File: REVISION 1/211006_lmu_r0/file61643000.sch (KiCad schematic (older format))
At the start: 7 parts

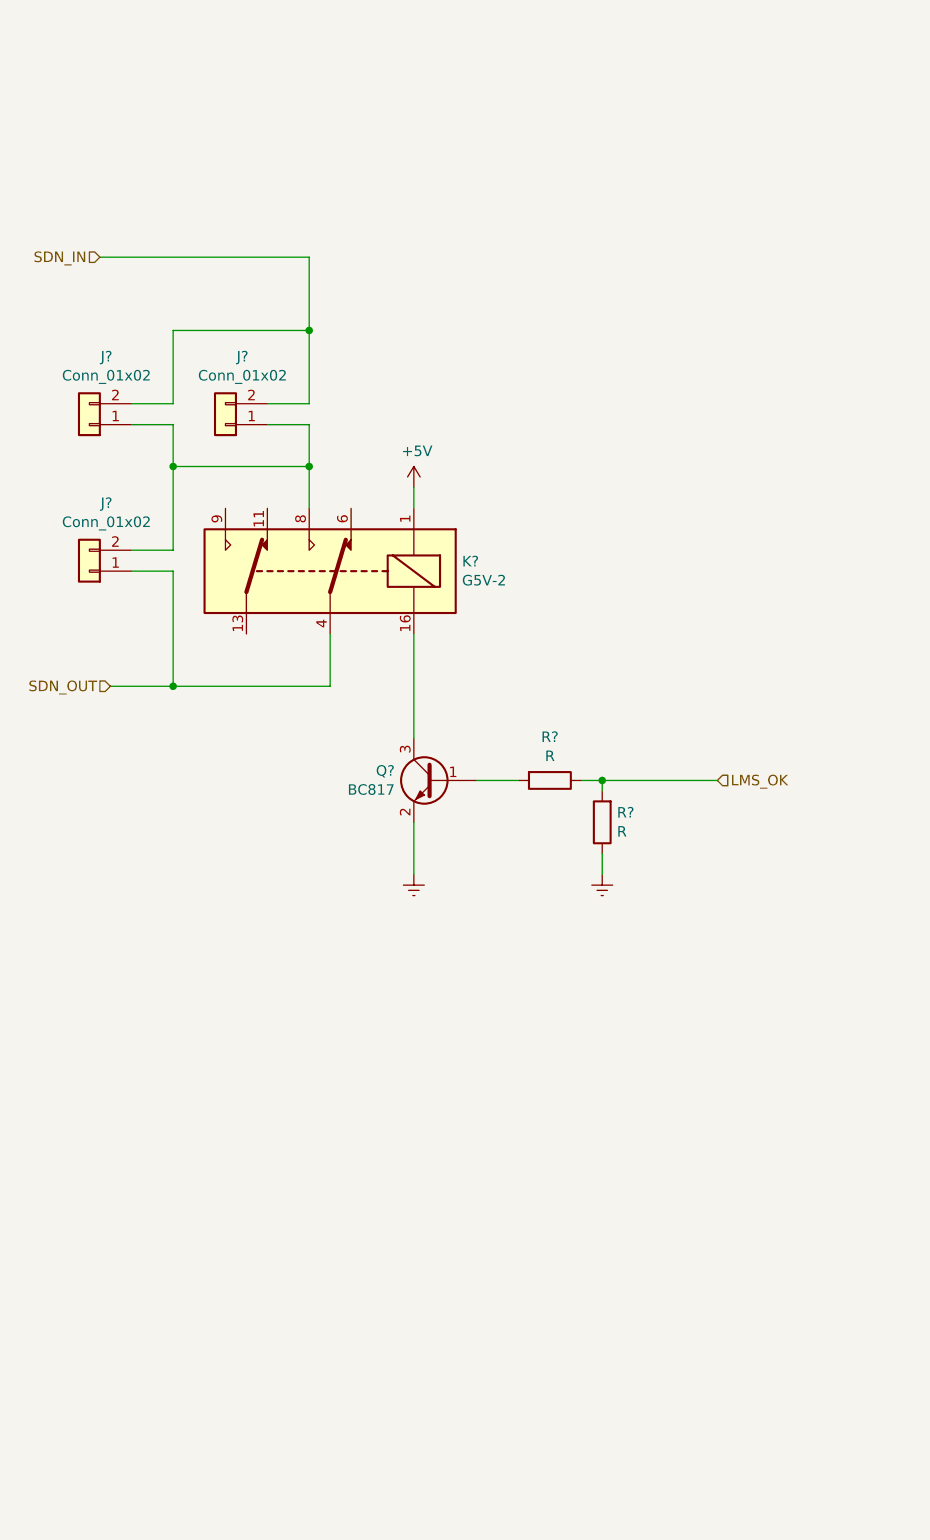
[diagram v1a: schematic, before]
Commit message: LMU design init
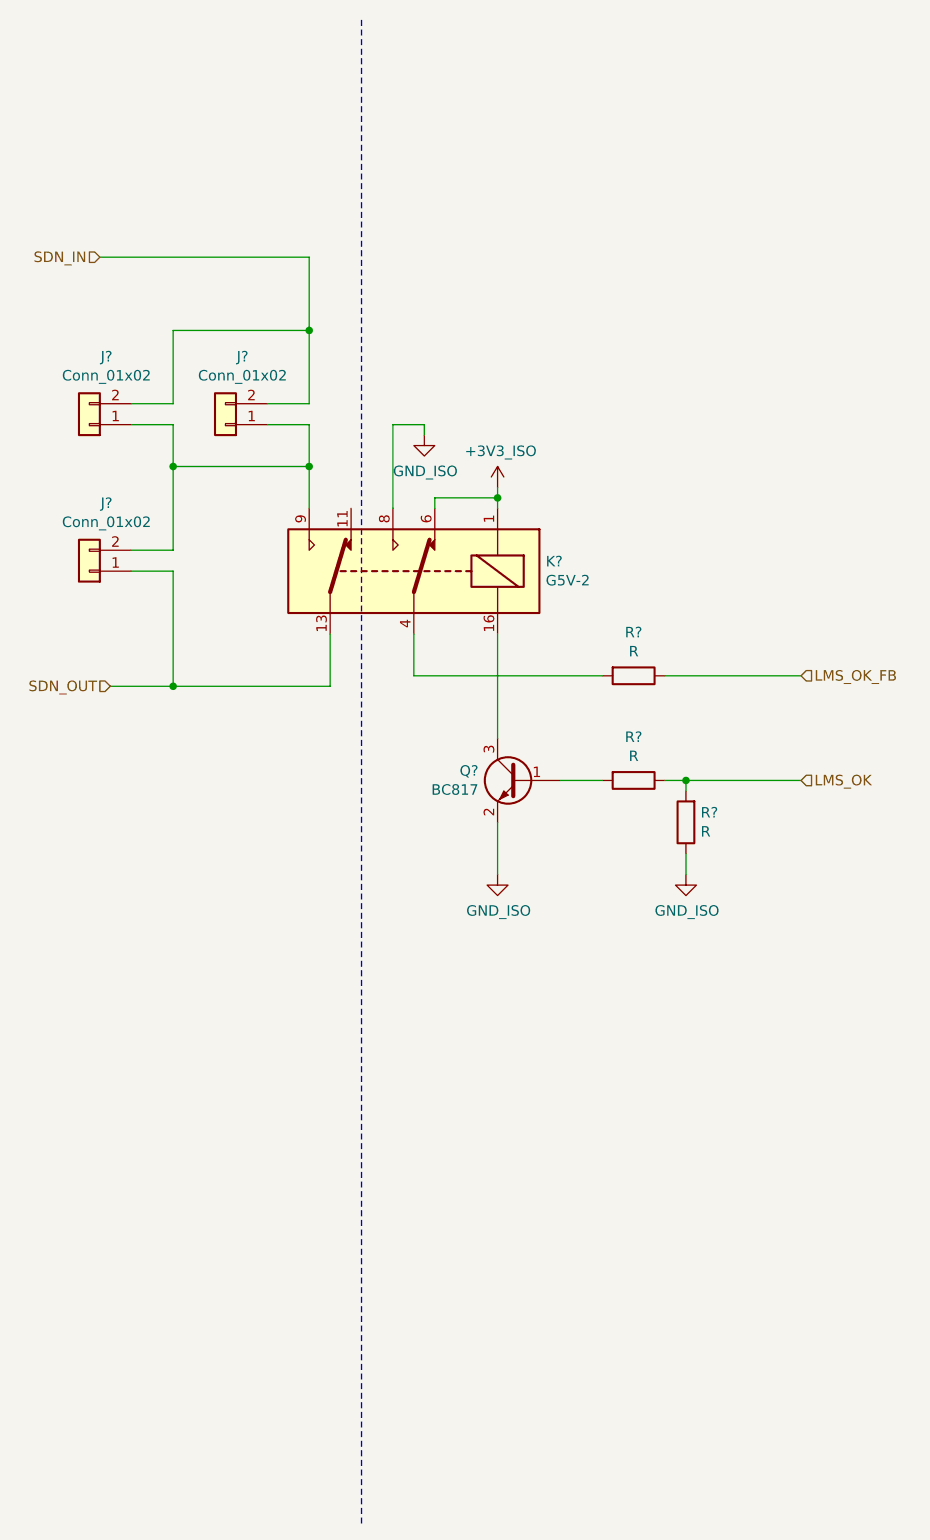
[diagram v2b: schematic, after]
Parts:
- added R?: R, symbol Device:R
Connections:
- net +5V is gone; now on net +3V3: K?.1
- net SDN_OUT: now also K?.13; no longer K?.4
- net +3V3: now reaches K?.6
- net at J?.1 (Pin_1), J?.1 (Pin_1), J?.2 (Pin_2): now also K?.9; no longer K?.8
- net Earth renamed GND
- net GND: now also K?.8
- new net: K?.4, R?.2
- new net LMS_OK_FB: R?.1
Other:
- moved on the sheet: K?, Q?, R?
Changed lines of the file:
@@
 $Descr A4 11693 8268
 encoding utf-8
-Sheet 4 30
+Sheet 30 30
 Title ""
 Date ""
@@
 L Transistor_BJT:BC817 Q?
 U 1 1 616435F7
-P 5650 4200
-F 0 "Q?" H 5841 4246 50  0000 L CNN
-F 1 "BC817" H 5841 4155 50  0000 L CNN
-F 2 "Package_TO_SOT_SMD:SOT-23" H 5850 4125 50  0001 L CIN
-F 3 "https://www.onsemi.com/pub/Collateral/BC818-D.pdf" H 5650 4200 50  0001 L CNN
-	1    5650 4200
+P 6050 4200
+F 0 "Q?" H 6241 4246 50  0000 L CNN
+F 1 "BC817" H 6241 4155 50  0000 L CNN
+F 2 "Package_TO_SOT_SMD:SOT-23" H 6250 4125 50  0001 L CIN
+F 3 "https://www.onsemi.com/pub/Collateral/BC818-D.pdf" H 6050 4200 50  0001 L CNN
+	1    6050 4200
 	-1   0    0    -1
 $EndComp
@@
 L Device:R R?
 U 1 1 61644D16
-P 6200 4200
-F 0 "R?" V 5993 4200 50  0000 C CNN
-F 1 "R" V 6084 4200 50  0000 C CNN
-F 2 "" V 6130 4200 50  0001 C CNN
-F 3 "~" H 6200 4200 50  0001 C CNN
-	1    6200 4200
+P 6600 4200
+F 0 "R?" V 6393 4200 50  0000 C CNN
+F 1 "R" V 6484 4200 50  0000 C CNN
+F 2 "" V 6530 4200 50  0001 C CNN
+F 3 "~" H 6600 4200 50  0001 C CNN
+	1    6600 4200
 	0    1    1    0
 $EndComp
-$Comp
-L Device:R R?
-U 1 1 6164548A
-P 6450 4400
-F 0 "R?" H 6380 4354 50  0000 R CNN
-F 1 "R" H 6380 4445 50  0000 R CNN
-F 2 "" V 6380 4400 50  0001 C CNN
-F 3 "~" H 6450 4400 50  0001 C CNN
-	1    6450 4400
-	-1   0    0    1
-$EndComp
-$Comp
-L power:Earth #PWR?
-U 1 1 616464DD
-P 6450 4650
-F 0 "#PWR?" H 6450 4400 50  0001 C CNN
-F 1 "Earth" H 6450 4500 50  0001 C CNN
-F 2 "" H 6450 4650 50  0001 C CNN
-F 3 "~" H 6450 4650 50  0001 C CNN
-	1    6450 4650
-	1    0    0    -1
-$EndComp
-Wire Wire Line
-	6450 4550 6450 4650
-Wire Wire Line
-	6350 4200 6450 4200
-Wire Wire Line
-	6450 4200 6450 4250
-Wire Wire Line
-	6050 4200 5850 4200
-$Comp
-L power:Earth #PWR?
-U 1 1 616470BA
-P 5550 4650
-F 0 "#PWR?" H 5550 4400 50  0001 C CNN
-F 1 "Earth" H 5550 4500 50  0001 C CNN
-F 2 "" H 5550 4650 50  0001 C CNN
-F 3 "~" H 5550 4650 50  0001 C CNN
-	1    5550 4650
-	1    0    0    -1
-$EndComp
-Wire Wire Line
-	5550 4400 5550 4650
+Wire Wire Line
+	6750 4200 6850 4200
+Wire Wire Line
+	6850 4200 6850 4250
+Wire Wire Line
+	6450 4200 6250 4200
+Wire Wire Line
+	5950 4400 5950 4650
 $Comp
 L Relay:G5V-2 K?
 U 1 1 61647A5A
-P 5150 3200
-F 0 "K?" H 4520 3246 50  0000 R CNN
-F 1 "G5V-2" H 4520 3155 50  0000 R CNN
-F 2 "Relay_THT:Relay_DPDT_Omron_G5V-2" H 5800 3150 50  0001 L CNN
-F 3 "http://omronfs.omron.com/en_US/ecb/products/pdf/en-g5v_2.pdf" H 5150 3200 50  0001 C CNN
-	1    5150 3200
+P 5550 3200
+F 0 "K?" H 4920 3246 50  0000 R CNN
+F 1 "G5V-2" H 4920 3155 50  0000 R CNN
+F 2 "Relay_THT:Relay_DPDT_Omron_G5V-2" H 6200 3150 50  0001 L CNN
+F 3 "http://omronfs.omron.com/en_US/ecb/products/pdf/en-g5v_2.pdf" H 5550 3200 50  0001 C CNN
+	1    5550 3200
 	-1   0    0    -1
 $EndComp
-$Comp
-L power:+5V #PWR?
-U 1 1 61649E5F
-P 5550 2800
-F 0 "#PWR?" H 5550 2650 50  0001 C CNN
-F 1 "+5V" H 5565 2973 50  0000 C CNN
-F 2 "" H 5550 2800 50  0001 C CNN
-F 3 "" H 5550 2800 50  0001 C CNN
-	1    5550 2800
-	1    0    0    -1
-$EndComp
-Wire Wire Line
-	5550 2800 5550 2900
-Wire Wire Line
-	5550 3500 5550 4000
-Wire Wire Line
-	6450 4200 7000 4200
-Connection ~ 6450 4200
-Text HLabel 7000 4200 2    50   Input ~ 0
+Wire Wire Line
+	5950 2800 5950 2850
+Wire Wire Line
+	5950 3500 5950 4000
+Wire Wire Line
+	6850 4200 7400 4200
+Connection ~ 6850 4200
+Text HLabel 7400 4200 2    50   Input ~ 0
 LMS_OK
 Text HLabel 4050 1700 0    50   Input ~ 0
@@
 Wire Wire Line
 	4400 3750 5150 3750
+Wire Wire Line
+	6850 4550 6850 4650
+$Comp
+L Device:R R?
+U 1 1 6164548A
+P 6850 4400
+F 0 "R?" H 6780 4354 50  0000 R CNN
+F 1 "R" H 6780 4445 50  0000 R CNN
+F 2 "" V 6780 4400 50  0001 C CNN
+F 3 "~" H 6850 4400 50  0001 C CNN
+	1    6850 4400
+	-1   0    0    1
+$EndComp
+$Comp
+L +3v3_iso:+3V3_ISO #PWR?
+U 1 1 616724FA
+P 5950 2800
+F 0 "#PWR?" H 5950 2650 50  0001 C CNN
+F 1 "+3V3_ISO" H 5965 2973 50  0000 C CNN
+F 2 "" H 5950 2800 50  0001 C CNN
+F 3 "" H 5950 2800 50  0001 C CNN
+	1    5950 2800
+	1    0    0    -1
+$EndComp
+$Comp
+L gnd_iso:GND_ISO #PWR?
+U 1 1 61672BF9
+P 5950 4650
+F 0 "#PWR?" H 5950 4400 50  0001 C CNN
+F 1 "GND_ISO" H 5955 4477 50  0000 C CNN
+F 2 "" H 5950 4650 50  0001 C CNN
+F 3 "" H 5950 4650 50  0001 C CNN
+	1    5950 4650
+	1    0    0    -1
+$EndComp
+$Comp
+L gnd_iso:GND_ISO #PWR?
+U 1 1 61673215
+P 6850 4650
+F 0 "#PWR?" H 6850 4400 50  0001 C CNN
+F 1 "GND_ISO" H 6855 4477 50  0000 C CNN
+F 2 "" H 6850 4650 50  0001 C CNN
+F 3 "" H 6850 4650 50  0001 C CNN
+	1    6850 4650
+	1    0    0    -1
+$EndComp
+Wire Notes Line
+	5300 7750 5300 550
+Wire Wire Line
+	5650 2900 5650 2850
+Wire Wire Line
+	5650 2850 5950 2850
+Connection ~ 5950 2850
+Wire Wire Line
+	5950 2850 5950 2900
+$Comp
+L Device:R R?
+U 1 1 61677209
+P 6600 3700
+F 0 "R?" V 6393 3700 50  0000 C CNN
+F 1 "R" V 6484 3700 50  0000 C CNN
+F 2 "" V 6530 3700 50  0001 C CNN
+F 3 "~" H 6600 3700 50  0001 C CNN
+	1    6600 3700
+	0    1    1    0
+$EndComp
+Wire Wire Line
+	6450 3700 5550 3700
+Wire Wire Line
+	5550 3700 5550 3500
+$Comp
+L gnd_iso:GND_ISO #PWR?
+U 1 1 616783FF
+P 5600 2550
+F 0 "#PWR?" H 5600 2300 50  0001 C CNN
+F 1 "GND_ISO" H 5605 2377 50  0000 C CNN
+F 2 "" H 5600 2550 50  0001 C CNN
+F 3 "" H 5600 2550 50  0001 C CNN
+	1    5600 2550
+	1    0    0    -1
+$EndComp
+Wire Wire Line
+	5450 2900 5450 2500
+Wire Wire Line
+	5450 2500 5600 2500
+Wire Wire Line
+	5600 2500 5600 2550
+Text HLabel 7400 3700 2    50   Input ~ 0
+LMS_OK_FB
+Wire Wire Line
+	7400 3700 6750 3700
 $EndSCHEMATC
